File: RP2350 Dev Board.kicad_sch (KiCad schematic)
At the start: 57 parts, among them J1 Conn_01x30_MountingPin, J2 Conn_01x30_MountingPin, U2 HC-1.0-3PWT, U4 ESP-PSRAM64H, U6 ESP-PSRAM32

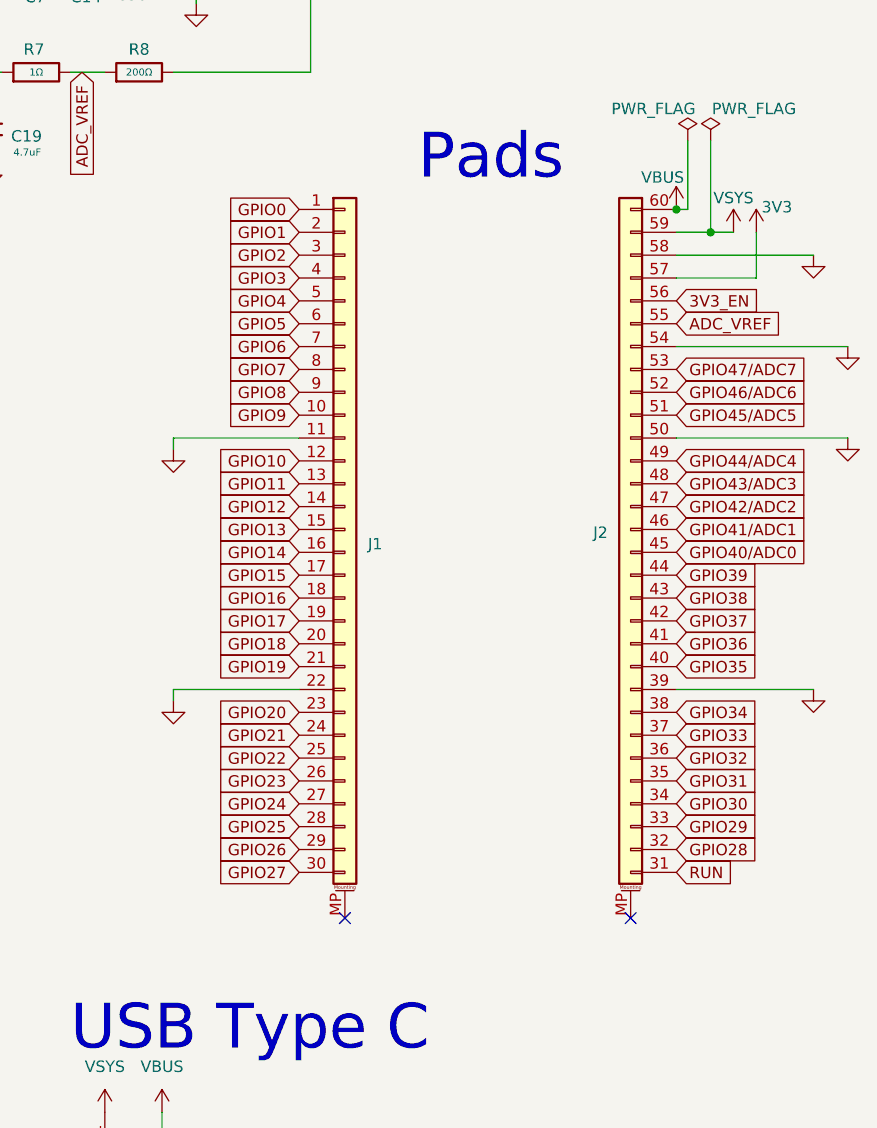
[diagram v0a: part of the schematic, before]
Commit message: Super version
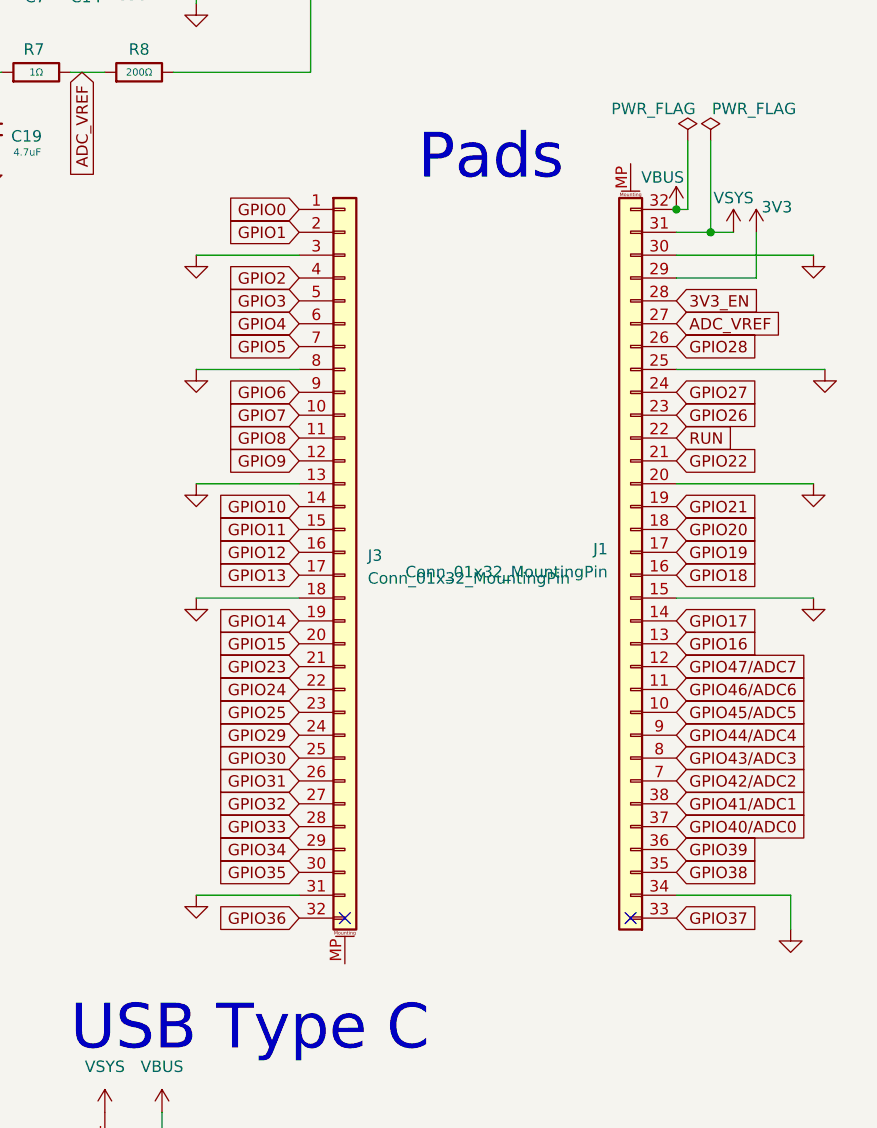
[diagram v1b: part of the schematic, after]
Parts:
- removed J1, J2: Conn_01x30_MountingPin, symbol Connector_Generic_MountingPin:Conn_01x30_MountingPin
- added J1, J3: Conn_01x32_MountingPin, symbol Connector_Generic_MountingPin:Conn_01x32_MountingPin
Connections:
- net 3V3: now also J1.29 (Pin_29)
- net 3V3_EN: now also J1.28 (Pin_28)
- net ADC_VREF: now also J1.27 (Pin_27)
- net GND: now also J1.15 (Pin_15), J1.20 (Pin_20), J1.25 (Pin_25), J1.30 (Pin_30), J1.34 (Pin_34), J3.13 (Pin_13), J3.18 (Pin_18), J3.3 (Pin_3), J3.31 (Pin_31), J3.8 (Pin_8)
- net GPIO0: now also J3.1 (Pin_1)
- net GPIO1: now also J3.2 (Pin_2)
- net GPIO10: now also J3.14 (Pin_14)
- net GPIO11: now also J3.15 (Pin_15)
- net GPIO12: now also J3.16 (Pin_16)
- net GPIO13: now also J3.17 (Pin_17)
- net GPIO14: now also J3.19 (Pin_19)
- net GPIO15: now also J3.20 (Pin_20)
- net GPIO16: now also J1.13 (Pin_13)
- net GPIO17: now also J1.14 (Pin_14)
- net GPIO18: now also J1.16 (Pin_16)
- net GPIO19: now also J1.17 (Pin_17)
- net GPIO2: now also J3.4 (Pin_4)
- net GPIO20: now also J1.18 (Pin_18)
- net GPIO21: now also J1.19 (Pin_19)
- net GPIO22: now also J1.21 (Pin_21)
- net GPIO23: now also J3.21 (Pin_21)
- net GPIO24: now also J3.22 (Pin_22)
- net GPIO25: now also J3.23 (Pin_23)
- net GPIO26: now also J1.23 (Pin_23)
- net GPIO27: now also J1.24 (Pin_24)
- net GPIO28: now also J1.26 (Pin_26)
- net GPIO29: now also J3.24 (Pin_24)
- net GPIO3: now also J3.5 (Pin_5)
- net GPIO30: now also J3.25 (Pin_25)
- net GPIO31: now also J3.26 (Pin_26)
- net GPIO32: now also J3.27 (Pin_27)
- net GPIO33: now also J3.28 (Pin_28)
- net GPIO34: now also J3.29 (Pin_29)
- net GPIO35: now also J3.30 (Pin_30)
- net GPIO36: now also J3.32 (Pin_32)
- net GPIO37: now also J1.33 (Pin_33)
- net GPIO38: now also J1.35 (Pin_35)
- net GPIO39: now also J1.36 (Pin_36)
- net GPIO4: now also J3.6 (Pin_6)
- net GPIO40/ADC0: now also J1.37 (Pin_37)
- net GPIO41/ADC1: now also J1.38 (Pin_38)
- net GPIO42/ADC2: now also J1.7 (Pin_7)
- net GPIO43/ADC3: now also J1.8 (Pin_8)
- net GPIO44/ADC4: now also J1.9 (Pin_9)
- net GPIO45/ADC5: now also J1.10 (Pin_10)
- net GPIO46/ADC6: now also J1.11 (Pin_11)
- net GPIO47/ADC7: now also J1.12 (Pin_12)
- net GPIO5: now also J3.7 (Pin_7)
- net GPIO6: now also J3.9 (Pin_9)
- net GPIO7: now also J3.10 (Pin_10)
- net GPIO8: now also J3.11 (Pin_11)
- net GPIO9: now also J3.12 (Pin_12)
- net RUN: now also J1.22 (Pin_22)
- net VBUS: now also J1.32 (Pin_32)
- net VSYS: now also J1.31 (Pin_31)
